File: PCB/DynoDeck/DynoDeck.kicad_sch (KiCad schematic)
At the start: 8 parts, among them J1 USB_C_Receptacle_USB2.0_16P, J2 E-paper, J3 CardKB, U1 E73-2G4M08S1C, U2 SX1262IMLTRT, U3 BQ25895RTW, U4 AMS1117-3.3, U5 TPS613222ADBV

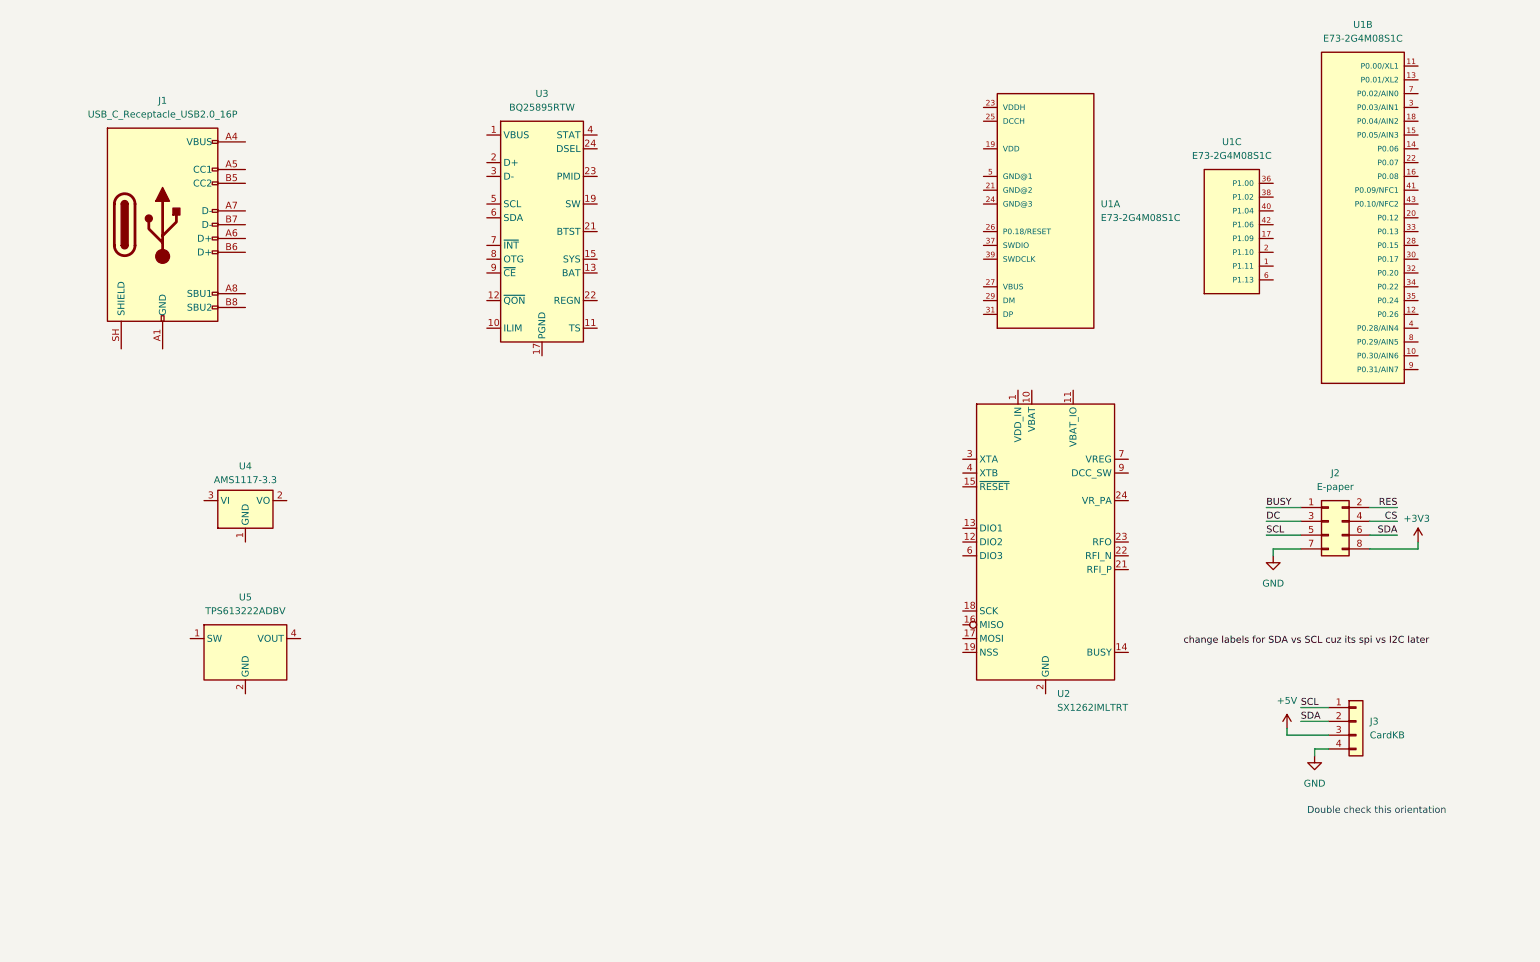
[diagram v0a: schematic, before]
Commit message: Schematic Power Circuit
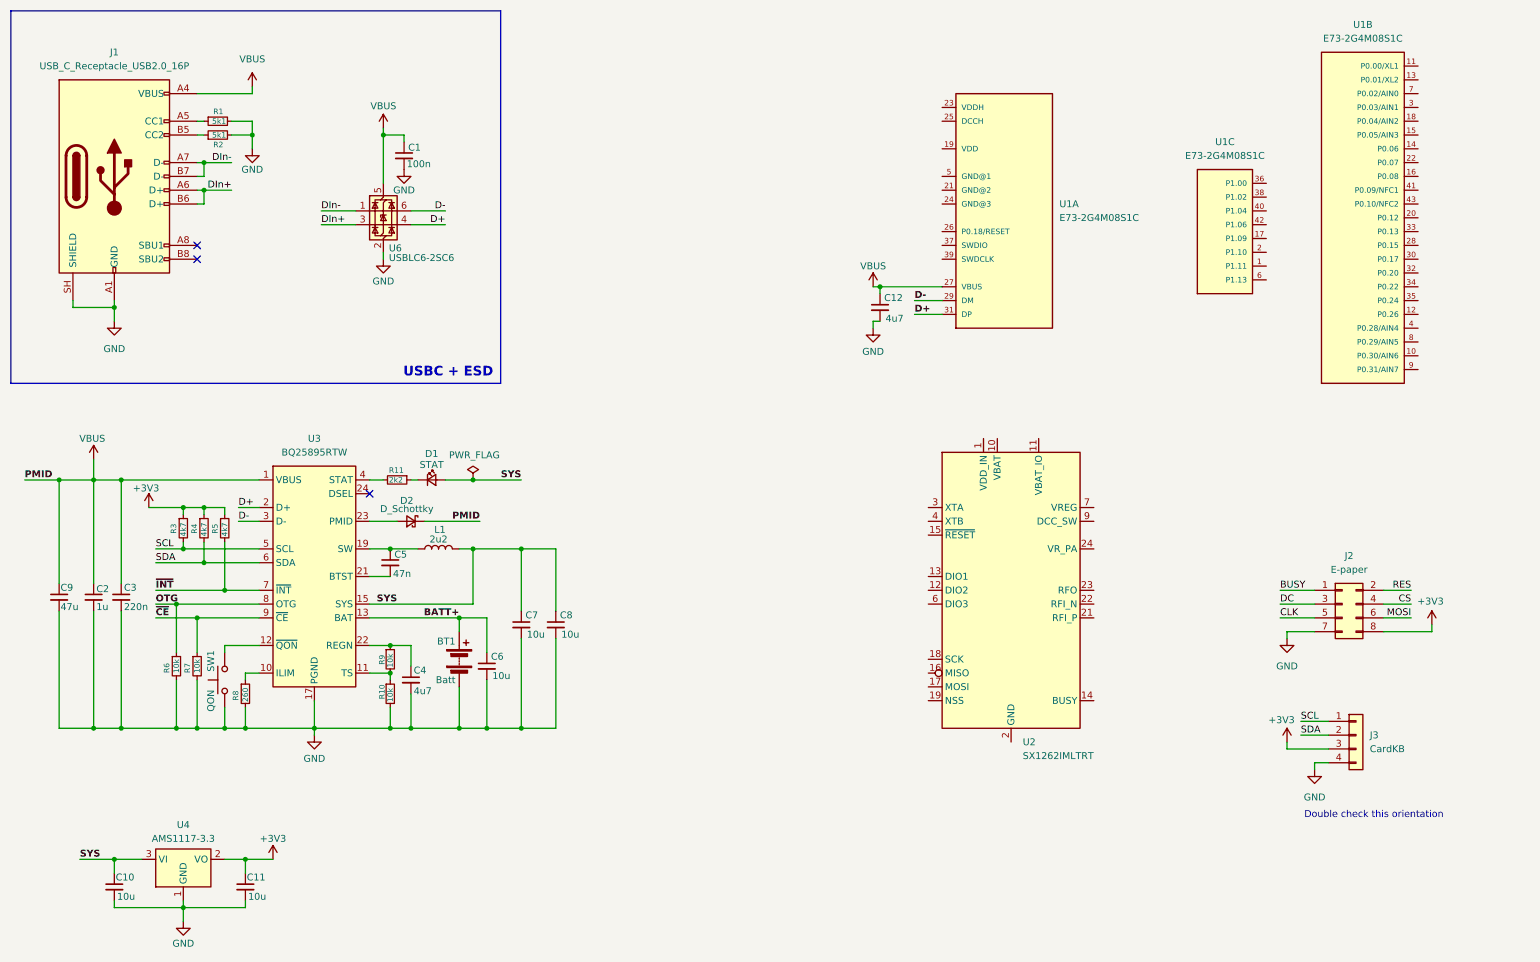
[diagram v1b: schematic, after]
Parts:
- removed U5: TPS613222ADBV, Package_TO_SOT_SMD:SOT-23-5, symbol Regulator_Switching:TPS613222ADBV
- added BT1: Batt, symbol Device:Battery
- added C1: 100n, symbol Device:C_Small
- added C10, C11, C6, C7, C8: 10u, symbol Device:C_Small
- added C12, C4: 4u7, symbol Device:C_Small
- added C2: 1u, symbol Device:C_Small
- added C3: 220n, symbol Device:C_Small
- added C5: 47n, symbol Device:C_Small
- added C9: 47u, symbol Device:C_Small
- added D1: STAT, symbol Device:LED_Small
- added D2: D_Schottky, symbol Device:D_Schottky_Small
- added L1: 2u2, symbol Device:L
- added R1, R2: 5k1, symbol Device:R_Small
- added R10, R6, R7, R9: 10k, symbol Device:R_Small
- added R11: 2k2, symbol Device:R_Small
- added R3, R4, R5: 4k7, symbol Device:R_Small
- added R8: 260, symbol Device:R_Small
- added SW1: QON, symbol Switch:SW_Push
- added U6: USBLC6-2SC6, Package_TO_SOT_SMD:SOT-23-6, symbol Power_Protection:USBLC6-2SC6
- J1: footprint (none) -> Connector_USB:USB_C_Receptacle_G-Switch_GT-USB-7010ASV
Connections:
- net +5V is gone; now on net +3V3: J3.3 (Pin_3)
- net +3V3: now also U4.2 (VO), C11.1, R3.1, R4.1, R5.1
- net GND: now also J1.A1 (GND), J1.A12 (GND), J1.B1 (GND), J1.B12 (GND), J1.SH (SHIELD), U3.17 (PGND), U3.18 (PGND), U3.25 (PGND), U4.1 (GND), BT1.2 (-), C1.2, C10.2, C11.2, C12.2, C2.2, C3.2, C4.2, C6.2, C7.2, C8.2, C9.2, R1.2, R10.2, R2.2, R6.2, R7.2, R8.2, SW1.2, U6.2 (GND)
- net SCL: now also U3.5 (SCL), R3.2; no longer J2.5 (Pin_5)
- net SDA: now also U3.6 (SDA), R4.2; no longer J2.6 (Pin_6)
- net VBUS: now reaches J1.A4 (VBUS), J1.A9 (VBUS), J1.B4 (VBUS), J1.B9 (VBUS)
- net VBUS: now also U1.27 (VBUS), U3.1 (VBUS), C1.1, C12.1, C2.1, C3.1, C9.1, D2.1 (K), U6.5 (VBUS)
- net at J1.A5 (CC1): now also R1.1
- net DIn+: now reaches J1.A6 (D+)
- net DIn+: now also J1.B6 (D+), U6.3 (I/O2)
- net DIn-: now reaches J1.A7 (D-)
- net DIn-: now also J1.B7 (D-), U6.1 (I/O1)
- net at J1.B5 (CC2): now also R2.1
- net D-: now reaches U1.29 (DM)
- net D-: now also U3.3 (D-), U6.6 (I/O1)
- net D+: now reaches U1.31 (DP)
- net D+: now also U3.2 (D+), U6.4 (I/O2)
- net SYS: now reaches U4.3 (VI)
- net SYS: now also U3.15 (SYS), U3.16 (SYS), C10.1, C7.1, C8.1, D1.2 (A), L1.2
- net at U3.10 (ILIM): now also R8.1
- net at U3.11 (TS): now also R10.1, R9.2
- net at U3.12 (~{QON}): now also SW1.1
- net BATT+: now reaches U3.13 (BAT), U3.14 (BAT)
- net BATT+: now also BT1.1 (+), C6.1
- net at U3.19 (SW), U3.20 (SW): now also C5.1, L1.1
- net at U3.21 (BTST): now also C5.2
- net at U3.22 (REGN): now also C4.1, R9.1
- net at U3.23 (PMID): now also D2.2 (A)
- net at U3.4 (STAT): now also R11.2
- net ~{INT}: now reaches U3.7 (~{INT})
- net ~{INT}: now also R5.2
- net OTG: now reaches U3.8 (OTG)
- net OTG: now also R6.1
- net ~{CE}: now reaches U3.9 (~{CE})
- net ~{CE}: now also R7.1
- new net: D1.1 (K), R11.1
- new net CLK: J2.5 (Pin_5)
- new net MOSI: J2.6 (Pin_6)
- no-connect marks 0 -> 3
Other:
- note added: "USBC + ESD"
- moved on the sheet: J1, J2, J3, U1A, U1C, U2, U3, U4
